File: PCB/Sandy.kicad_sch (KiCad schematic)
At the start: 151 parts, among them J1 USB_C_Receptacle_USB2.0, J16 Conn_01x04, J18 Conn_01x04, J2 Conn_01x03, J3 Conn_01x02, J4 Conn_02x04_Top_Bottom, J5 Conn_02x03_Odd_Even, J6 Conn_02x04_Top_Bottom, J7 Conn_02x04_Top_Bottom, J8 Conn_02x04_Top_Bottom, U1 ATmega32U4-MU, U2 24LC64, Y1 16MHz

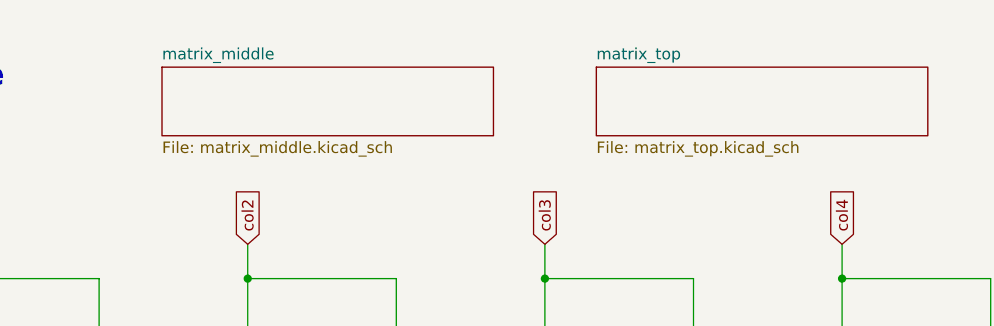
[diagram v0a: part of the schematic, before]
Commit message: MCUさっくり配置
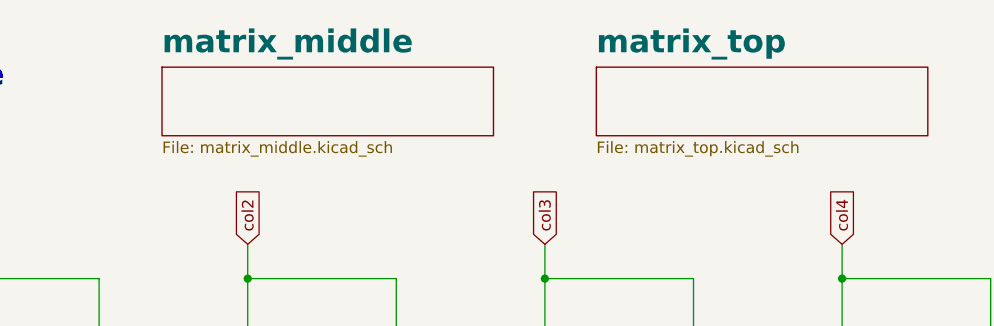
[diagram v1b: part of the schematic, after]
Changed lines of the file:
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@@
     (stroke (width 0.1524) (type solid) (color 0 0 0 0))
     (fill (color 0 0 0 0.0000))
-    (property "Sheet name" "matrix_middle" (id 0) (at 80.01 17.0684 0)
-      (effects (font (size 1.27 1.27)) (justify left bottom))
+    (property "Sheet name" "matrix_middle" (id 0) (at 80.01 16.4334 0)
+      (effects (font (size 2.54 2.54) bold) (justify left bottom))
     )
     (property "Sheet file" "matrix_middle.kicad_sch" (id 1) (at 80.01 25.9846 0)
@@
     (stroke (width 0.1524) (type solid) (color 0 0 0 0))
     (fill (color 0 0 0 0.0000))
-    (property "Sheet name" "matrix_top" (id 0) (at 128.27 17.0684 0)
-      (effects (font (size 1.27 1.27)) (justify left bottom))
+    (property "Sheet name" "matrix_top" (id 0) (at 128.27 16.4334 0)
+      (effects (font (size 2.54 2.54) bold) (justify left bottom))
     )
     (property "Sheet file" "matrix_top.kicad_sch" (id 1) (at 128.27 25.9846 0)
